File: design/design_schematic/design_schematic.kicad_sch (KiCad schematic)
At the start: 145 parts, among them IC1 XC9291B33D0R-G, IC2 XC9148G50CER-G, IC4 74AHCT125PW,118, J1 USB_C_Receptacle_USB2.0_16P, J2 Battery Pos, J3 Battery Neg, J4 OLED_128x32, J5 0781271220, J6 Conn_01x05, SW1 SW_SPST, SW2 SW_Push, U1 nRF52840, U2 BQ24072RGT, U3 USB6B1, U4 BQ27441-G1, U5 PEC11L-4015F-S0015, U6 PEC11L-4015F-S0015, X1 32MHz

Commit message: vbus routing
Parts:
- removed C37, C40, C43, C49: 100nF, ScottoKeebs_Components:Capacitor_0402, symbol Device:C_Small
- removed C46: 10uF, ScottoKeebs_Components:Capacitor_0402, symbol Device:C_Small
- removed J6: Conn_01x05, symbol Connector_Generic:Conn_01x05
- removed L3: 10uH, Inductor_SMD:L_0402_1005Metric, symbol Device:L_Small
- removed L4: 10uH, Inductor_SMD:L_0201_0603Metric, symbol Device:L_Small
- removed R13: 10k, symbol Device:R
- removed SW1: SW_SPST, symbol Switch:SW_SPST
- removed SW2: SW_Push, symbol Switch:SW_Push
- removed U1: nRF52840, Package_DFN_QFN:Nordic_AQFN-73-1EP_7x7mm_P0.5mm, symbol MCU_Nordic:nRF52840
- added C29, C30, C32, C33: 100nF, ScottoKeebs_Components:Capacitor_0603, symbol Device:C_Small
- added C35: 22uF, ScottoKeebs_Components:Capacitor_0603, symbol Device:C_Small
- added IC3: nRF52833-QDAA-R7, SamacSys_Parts:QFN40P500X500X90-41N-D, symbol SamacSys_Parts:nRF52833-QDAA-R7
- added IC5: MCP23018T-E_SS, SamacSys_Parts:SOP65P780X200-24N, symbol SamacSys_Parts:MCP23018T-E_SS
- added IC6: XC9291B33D1R-G, XC9290A07E1RG, symbol SamacSys_Parts:XC9291B33D1R-G
- added J6: Conn_01x04, symbol Connector_Generic:Conn_01x04
- added S26: CL-SA-12C4-22, SamacSys_Parts:CLSA12C422, symbol SamacSys_Parts:CL-SA-12C4-22
- C1, C2: value 12pF -> 4.7uF; footprint ScottoKeebs_Components:Capacitor_0402 -> ScottoKeebs_Components:Capacitor_0603
- C10, C13, C17, C18, C22, C23, C24, C25, C26, C27, C28, C31, C7, C8, C9: footprint ScottoKeebs_Components:Capacitor_0402 -> ScottoKeebs_Components:Capacitor_0603
- C11: value 100pF -> 820pF; footprint ScottoKeebs_Components:Capacitor_0402 -> ScottoKeebs_Components:Capacitor_0603
- C12: value 100nF -> 100pF; footprint ScottoKeebs_Components:Capacitor_0402 -> ScottoKeebs_Components:Capacitor_0603
- C14: value 1uF -> 12pF
- C15: value 1uF -> 1.2pF
- C16: value 47nF -> 1pF; footprint ScottoKeebs_Components:Capacitor_0402 -> ScottoKeebs_Components:Capacitor_0603
- C19: value 4.7uF -> 12pF
- C20, C21: value 4.7uF -> 100nF
- C3: value 0.8pF -> 100nF; footprint ScottoKeebs_Components:Capacitor_0402 -> ScottoKeebs_Components:Capacitor_0603
- C34: value 100nF -> 10uF; footprint ScottoKeebs_Components:Capacitor_0402 -> ScottoKeebs_Components:Capacitor_0603
- C4: value 0.5pF -> 4.7uF; footprint ScottoKeebs_Components:Capacitor_0402 -> ScottoKeebs_Components:Capacitor_0603
- C5: value 100nF -> 1uF; footprint ScottoKeebs_Components:Capacitor_0402 -> ScottoKeebs_Components:Capacitor_0603
- C6: value 4.7uF -> 1uF
- F1: footprint (none) -> SamacSys_Parts:0603L050SLYR
- IC2: footprint (none) -> SamacSys_Parts:XC9147_8_USP-6C
- J2, J3: footprint (none) -> Connector_Wire:SolderWire-2.5sqmm_1x01_D2.4mm_OD3.6mm
- L1: footprint Inductor_SMD:L_0402_1005Metric -> Inductor_SMD:L_0603_1608Metric
- L2: value 15nH -> 2.2nH; footprint Inductor_SMD:L_0201_0603Metric -> Inductor_SMD:L_0603_1608Metric
- L5, L6: footprint (none) -> Inductor_SMD:L_0603_1608Metric
- R1, R10, R11, R12, R2, R3, R4, R5, R6, R7, R8, R9: footprint (none) -> Resistor_SMD:R_0603_1608Metric
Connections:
- net VDD_HV is gone; now on net GND: C19.2
- net 2A: now also IC3.23 (P0.10)
- net 3V3: now also C1.2, C20.2, C5.1, C7.1, C8.1, IC3.18 (VDD_2), IC3.30 (VDD_3), IC3.40 (VDD_4), IC3.8 (VDD_1), IC3.9 (VDDH), IC5.10 (VDD), J6.1 (Pin_1); no longer C12.2, C14.2, C6.2, C7.2, C8.2
- net 5V: now also C21.1, C29.1, C30.1, C32.1, C33.1
- net CCW: now also IC3.15 (P0.17)
- net CCW2: now also IC3.16 (P0.18)
- net CHG: now also IC5.19 (GPA2)
- net CW: now also IC3.14 (P0.15)
- net CW2: now also IC3.17 (P0.20)
- net Column 0: now also IC3.36 (P0.31)
- net Column 1: now also IC3.35 (P0.30)
- net Column 2: now also IC3.34 (P0.29)
- net Column 3: now also IC3.33 (P0.28)
- net Column 4: now also IC3.32 (P0.02)
- net Column 5: now also IC3.31 (P0.03)
- net D+: now also IC3.13 (D+)
- net D-: now also IC3.12 (D-)
- net GND: now also C11.2, C12.2, C14.2, C16.1, C2.1, C21.2, C3.1, C5.2, C7.2, C8.2, C29.2, C30.2, C32.2, C33.2, C35.2, IC3.25 (VSS_PA), IC3.37 (VSS_1), IC3.41 (VSS_2), IC5.1 (VSS), J6.2 (Pin_2); no longer C11.1, C12.1, C14.1, C16.2, C19.1, C2.2, C21.1, C3.2, C5.1, C7.1, C8.1
- net NO: now also IC5.17 (GPA0)
- net NO2: now also IC5.18 (GPA1)
- net Row 0: now also IC3.4 (P0.04)
- net Row 1: now also IC3.5 (P0.05)
- net Row 2: now also IC3.6 (P1.09)
- net Row 3: now also IC3.7 (P0.11)
- net SCL: now also R10.1, IC3.2 (P0.00), IC5.11 (SCL); no longer R11.1
- net SDA: now also R11.1, IC3.3 (P0.01), IC5.12 (SDA); no longer R10.1
- net VBUS: now also C2.2, C23.2, F1.2, U2.13 (IN), U2.6 (EN1), U3.1 (VBUS), U3.8 (VBUS), C35.1, IC3.10 (VBUS); no longer C21.2
- net at L2.2: now also C15.1, L1.2
- net at X1.1: now also C14.1, IC3.29 (XC2); no longer C2.1
- net at X1.2: now also C19.1, IC3.28 (XC1); no longer C1.2
- net at D11.4 (DIN): now also D15.2 (DOUT); no longer D10.2 (DOUT)
- net at D10.4 (DIN): now also D6.2 (DOUT); no longer D9.2 (DOUT)
- net at D13.2 (DOUT): now also D17.4 (DIN); no longer D14.4 (DIN)
- net at D13.4 (DIN): now also D9.2 (DOUT); no longer D12.2 (DOUT)
- net at D24.4 (DIN): now also D22.2 (DOUT); no longer D23.2 (DOUT)
- net at D23.4 (DIN): now also D21.2 (DOUT); no longer D22.2 (DOUT)
- net at C10.1, C25.1, IC1.1 (EN)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: now also S26.1 (COM)
- net at D8.2 (DOUT): now also D4.4 (DIN); no longer D9.4 (DIN)
- net at D7.2 (DOUT): now also D3.4 (DIN); no longer D8.4 (DIN)
- net at D7.4 (DIN): now also D11.2 (DOUT); no longer D6.2 (DOUT)
- net at L1.1: now also C16.2, IC3.24 (ANT); no longer C4.2
- net at D22.4 (DIN): now also D18.2 (DOUT); no longer D21.2 (DOUT)
- net at D21.4 (DIN): now also D17.2 (DOUT); no longer D20.2 (DOUT)
- net at D16.4 (DIN): now also D20.2 (DOUT); no longer D15.2 (DOUT)
- net at D15.4 (DIN): now also D19.2 (DOUT); no longer D14.2 (DOUT)
- net at D16.2 (DOUT): now also D12.4 (DIN); no longer D17.4 (DIN)
- net at D19.4 (DIN): now also D23.2 (DOUT); no longer D18.2 (DOUT)
- net at D18.4 (DIN): now also D14.2 (DOUT); no longer D17.2 (DOUT)
- net at D2.4 (DIN): now also D3.2 (DOUT); no longer D1.2 (DOUT)
- net at D20.4 (DIN): now also D24.2 (DOUT); no longer D19.2 (DOUT)
- net at D2.2 (DOUT): now also D6.4 (DIN); no longer D3.4 (DIN)
- net at U2.10 (OUT), U2.11 (OUT): now also S26.2 (NO)
- net at D5.2 (DOUT): now also D9.4 (DIN); no longer D6.4 (DIN)
- net at D5.4 (DIN): now also D1.2 (DOUT); no longer D4.2 (DOUT)
- new net: C3.2, IC3.1 (DEC1)
- new net: C11.1, IC3.21 (DEC5)
- new net: D12.2 (DOUT), D8.4 (DIN)
- new net: C4.2, IC3.11 (DECUSB)
- new net: IC3.19 (SWDIO), J6.4 (Pin_4)
- new net: IC3.20 (SWDCLK), J6.3 (Pin_3)
- new net: C12.1, IC3.27 (DEC3)
- new net: D10.2 (DOUT), D14.4 (DIN)
- new net DEC4: C6.2, IC3.26 (DEC6), IC3.38 (DEC4)
- new net INTA: IC3.22 (P0.09), IC5.16 (INTA)
- new net RF: L2.1
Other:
- note added: "GPIO Expander"
- note added: "nRF52833 Module"
- note removed: "nRF52840 Module"
- moved on the sheet: C25

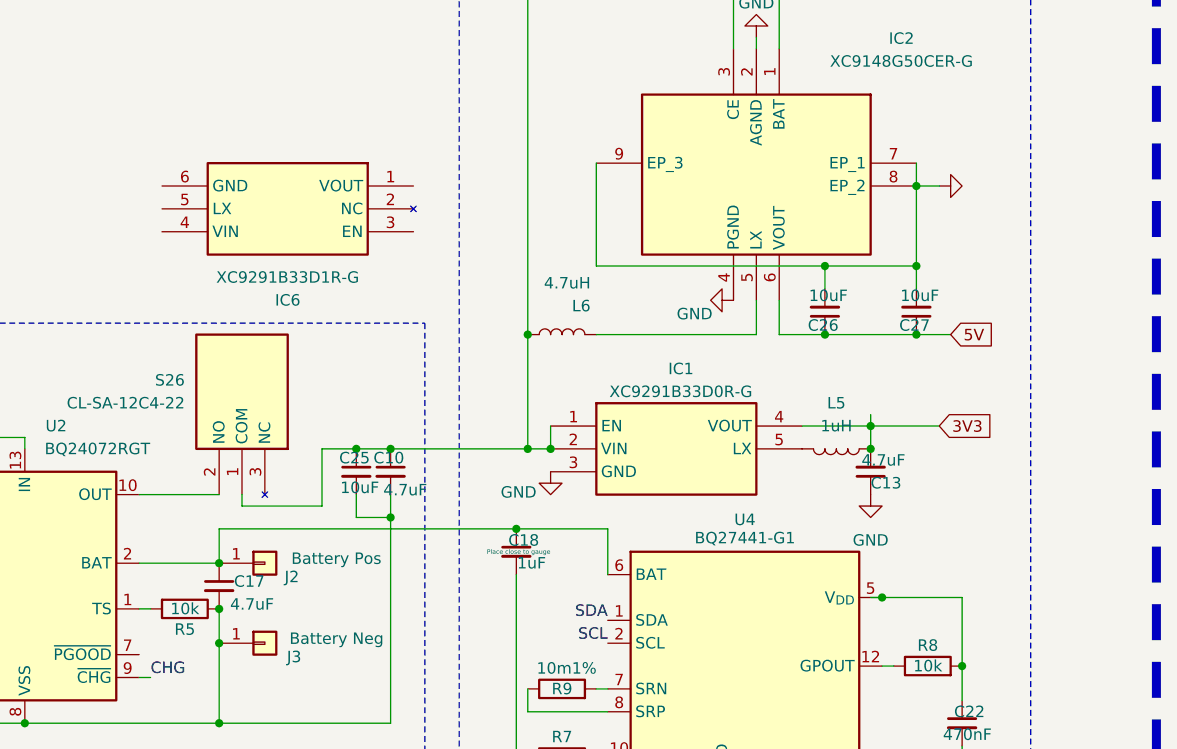
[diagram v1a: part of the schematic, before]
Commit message: prepare to change switch footprint
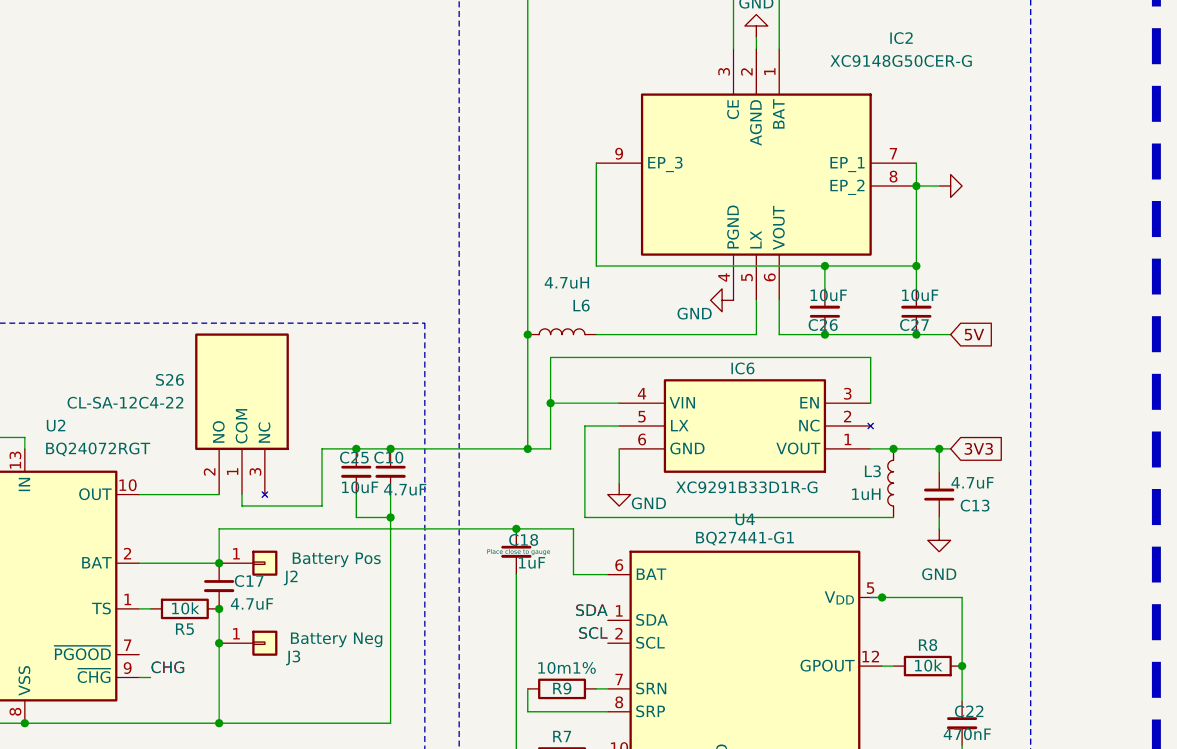
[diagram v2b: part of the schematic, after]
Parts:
- removed IC1: XC9291B33D0R-G, SamacSys_Parts:XC9290A07E0RG, symbol SamacSys_Parts:XC9291B33D0R-G
- removed L5: 1uH, Inductor_SMD:L_0603_1608Metric, symbol Device:L
- added L3: 1uH, Inductor_SMD:L_0603_1608Metric, symbol Device:L
- IC6: footprint XC9290A07E1RG -> SamacSys_Parts:XC9290A07E1RG
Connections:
- net 3V3: now also IC6.1 (VOUT), L3.1
- net GND: now also IC6.6 (GND)
- net at C10.1, C25.1, IC2.1 (BAT)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: now also IC6.3 (EN), IC6.4 (VIN)
- net at IC6.5 (LX): now also L3.2
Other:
- moved on the sheet: IC6
